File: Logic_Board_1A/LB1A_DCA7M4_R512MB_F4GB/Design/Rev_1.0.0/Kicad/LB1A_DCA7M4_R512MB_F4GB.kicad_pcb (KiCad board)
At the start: 6 copper layers, 50 x 50 mm, 143 parts, among them U1 STM32MP157CAC3, U2 AS4C256M16D3LC-12BCN, U3 S40FC004C1B2C00000, U4 STPMIC1BPQR, U5 DF40C-70DP-0.4V(51), U6 DF40C-70DP-0.4V(51), U7 DF40C-70DP-0.4V(51), X1 32.768kHz, X2 24MHz

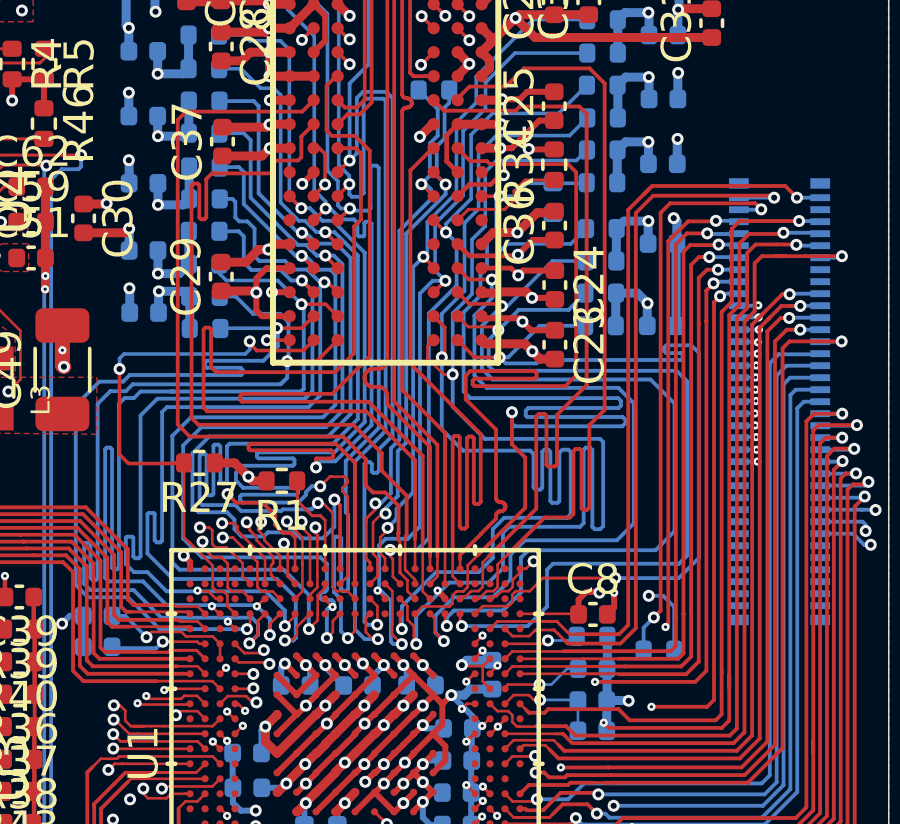
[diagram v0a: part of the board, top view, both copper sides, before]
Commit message: more improvements on PCB
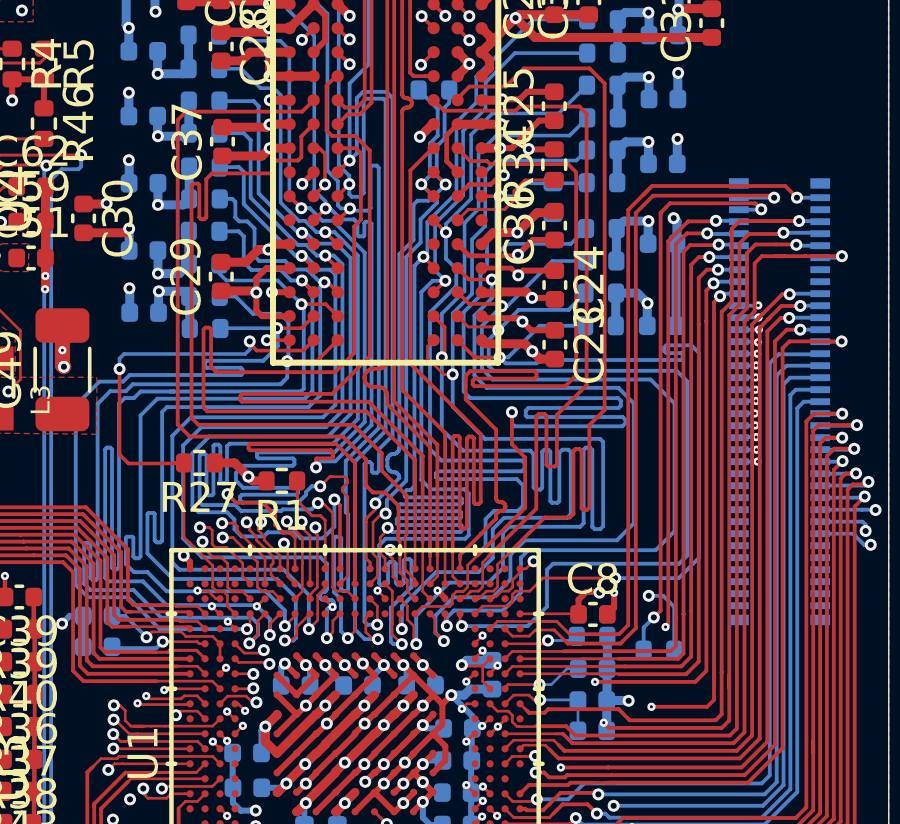
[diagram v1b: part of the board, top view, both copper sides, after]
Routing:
- net DDR_A12: track 22.9 -> 35.5 mm
- net DDR_A10: track 22.2 -> 33.7 mm
- net DDR_A1: track 28.2 -> 35.5 mm
- net DDR_CLK_N: track 18.4 -> 18.9 mm

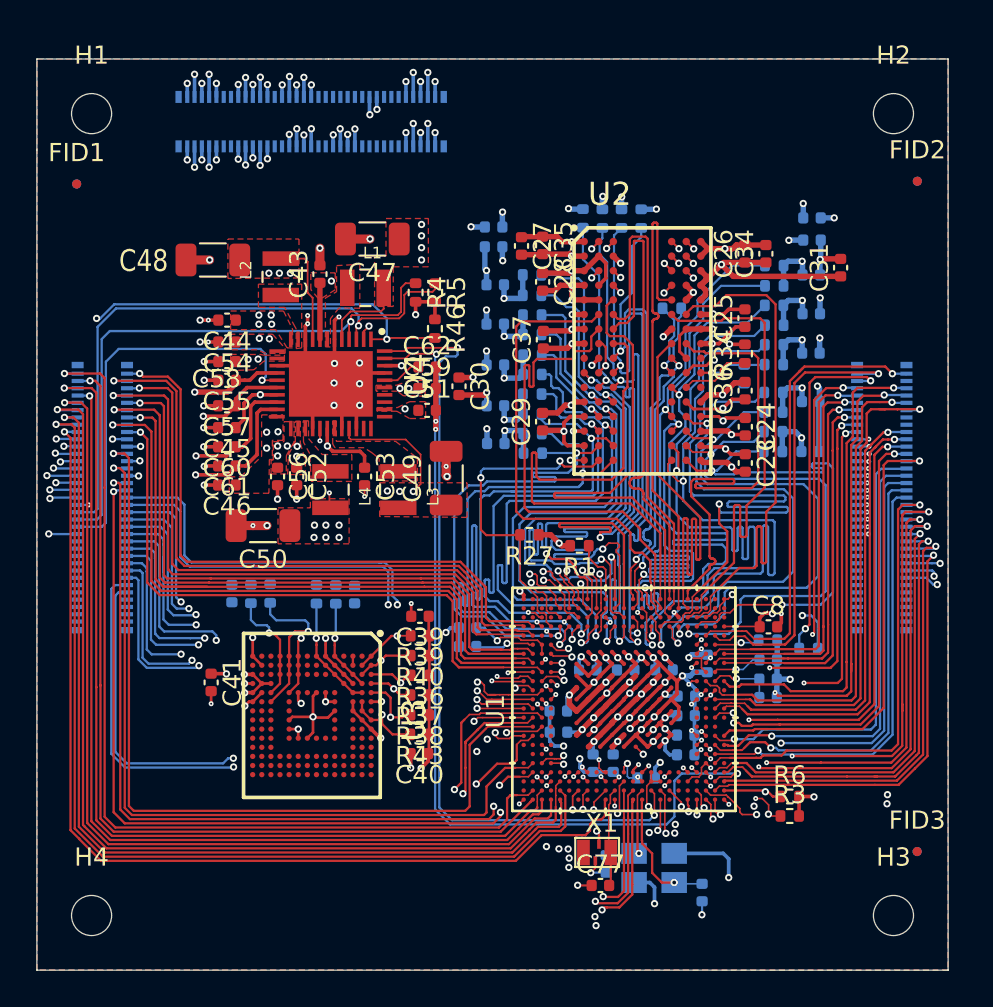
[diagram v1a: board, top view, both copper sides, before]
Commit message: improvements
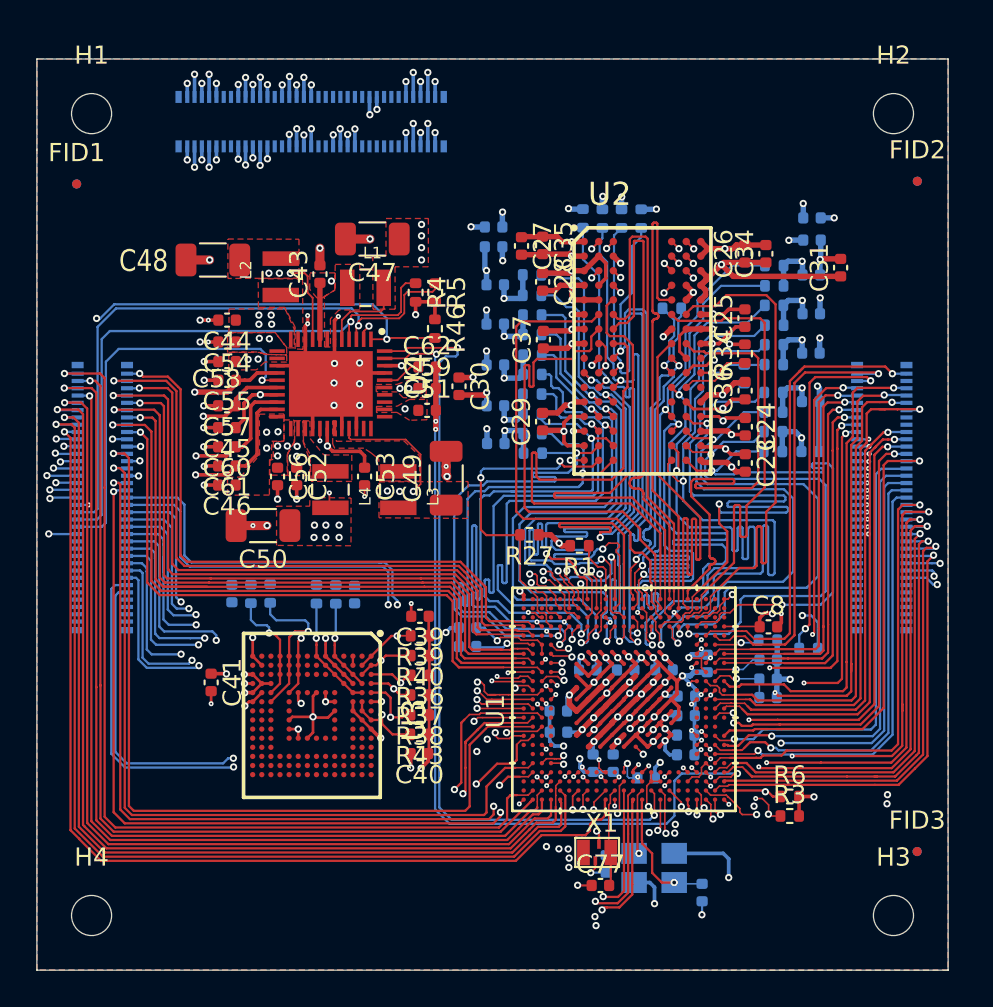
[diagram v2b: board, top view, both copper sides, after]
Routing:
- net PMIC_VOUT2_VDD_DDR: track 55.6 -> 54.3 mm
- net USART1_TX: track 25.8 -> 26.6 mm
- removed copper zone on Signal_Layer_3.Cu, net PMIC_LDO5_2V9
- removed copper zone on Signal_Layer_3.Cu, net PMIC_VOUT3_VDD
- removed copper zone on Signal_Layer_4.Cu, net PMIC_VOUT4_3V3
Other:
- net class DDR_DiffPairs: clearance 0.1016 -> 0.0762
- net class Default: clearance 0.1016 -> 0.0762
- net class Gnd_Lines: clearance 0.1016 -> 0.0762
- rule trace_clearance: 0.1016 -> 0.0762
